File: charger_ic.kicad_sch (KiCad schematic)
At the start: 1 part, among them U8 BQ25731RSNR

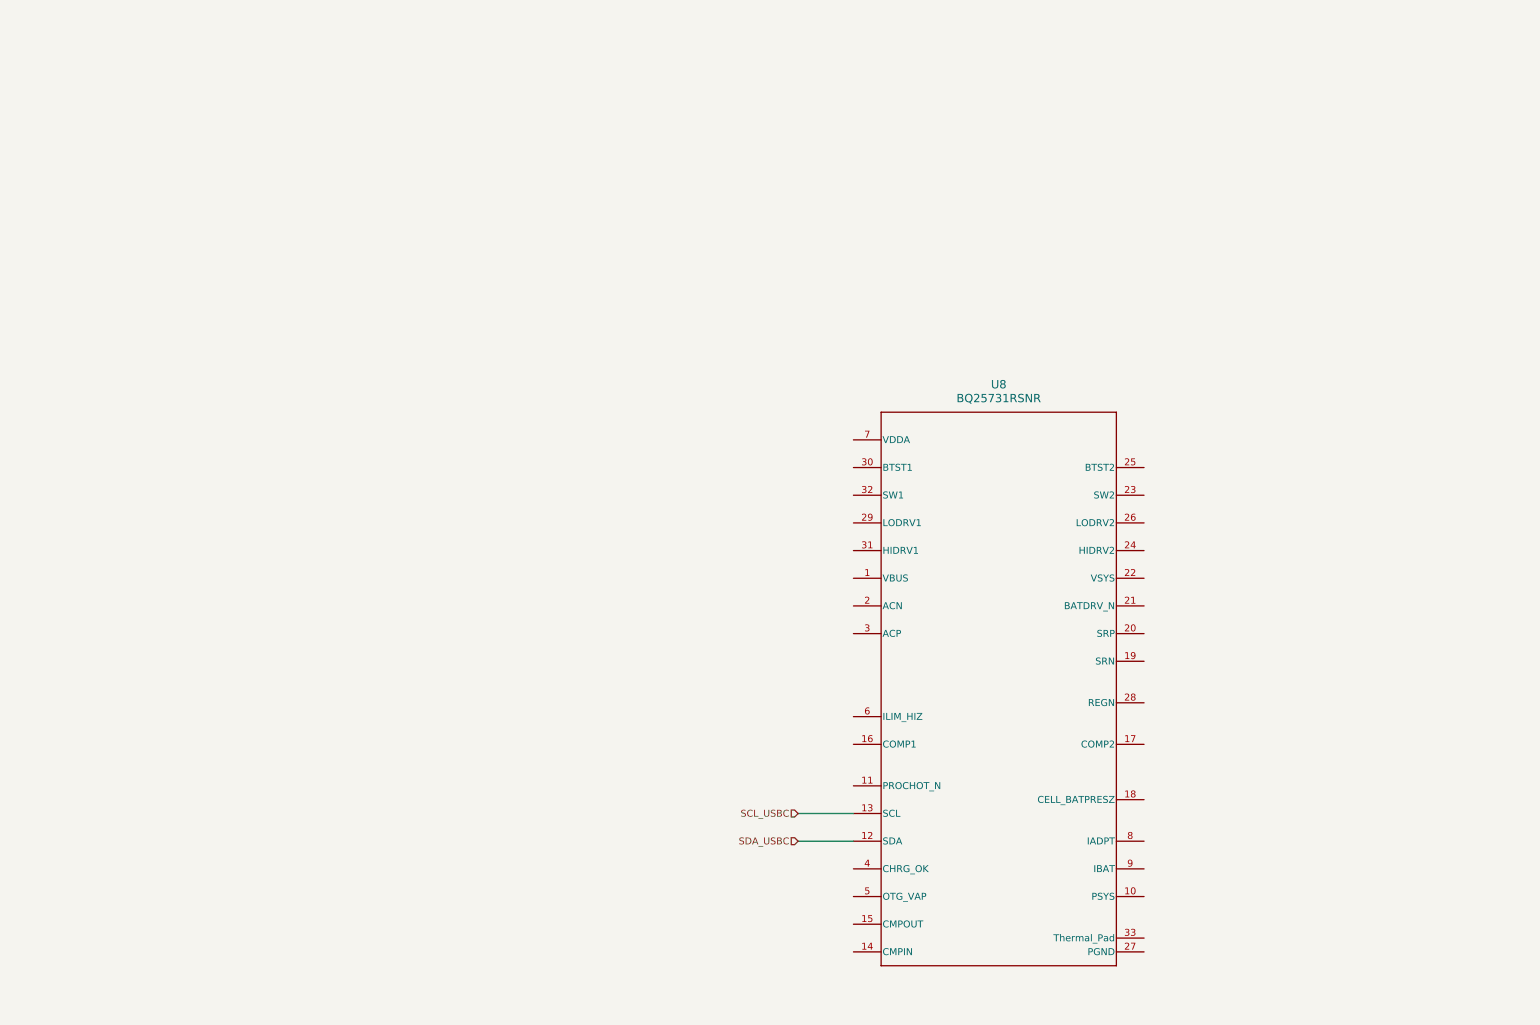
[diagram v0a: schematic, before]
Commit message: adding charging stages finally
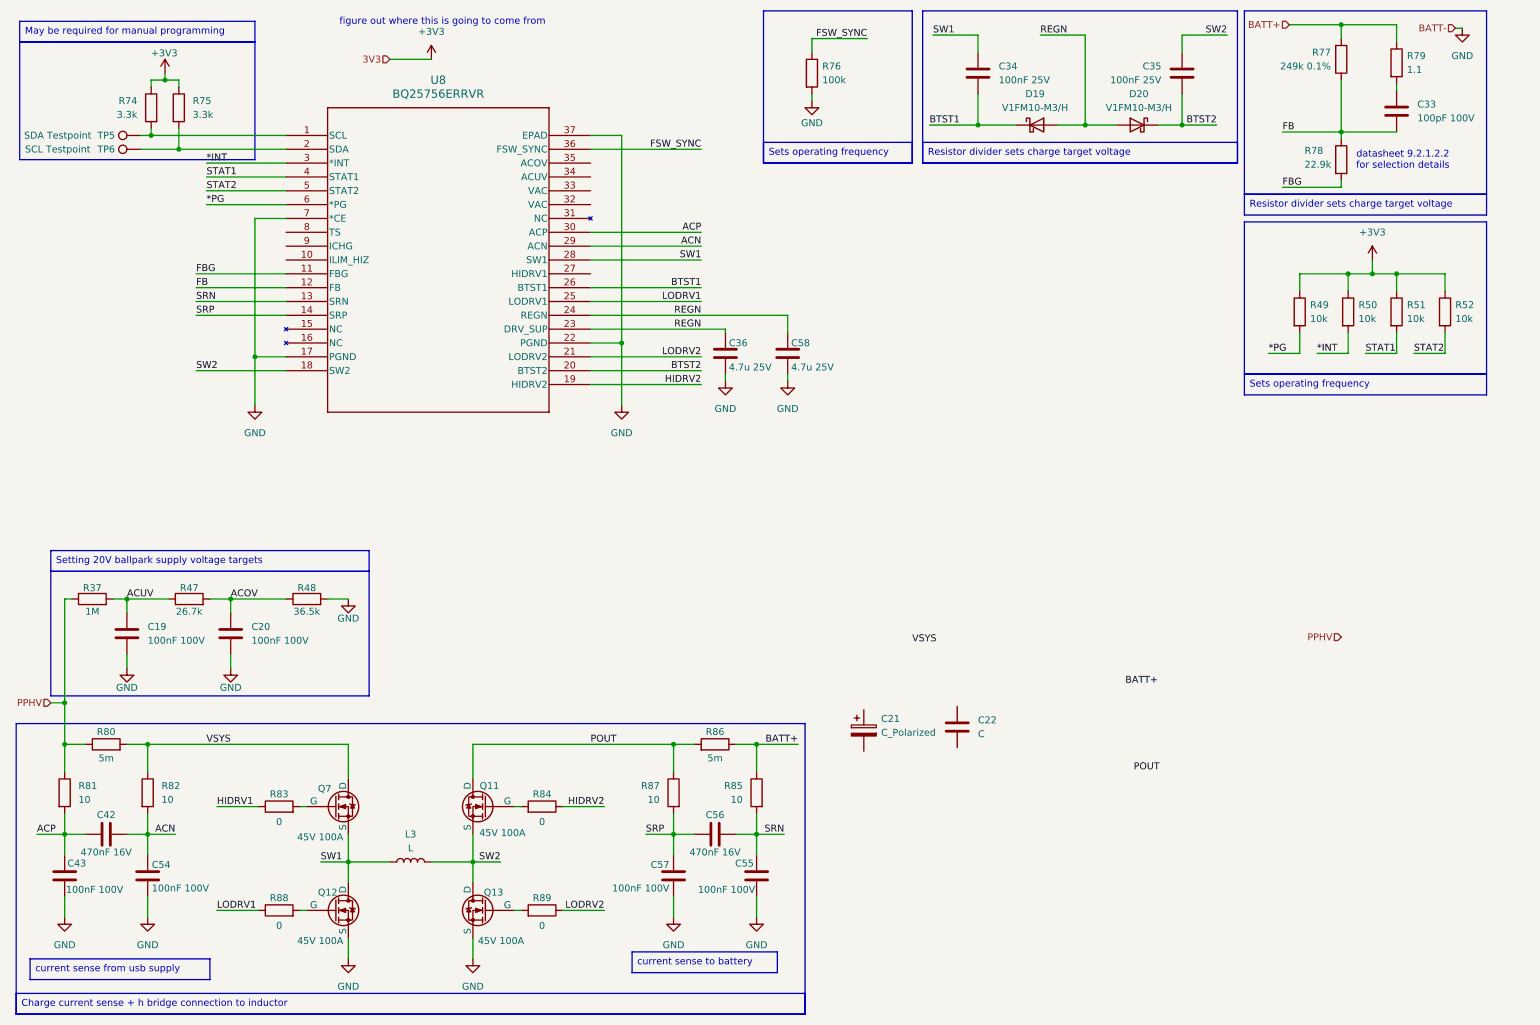
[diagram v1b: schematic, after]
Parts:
- removed U8: BQ25731RSNR, RSN0032B-IPC_A, symbol BQ25731:BQ25731RSNR
- added C19, C20, C43, C54, C55, C57: 100nF 100V, symbol Device:C
- added C21: C_Polarized, symbol Device:C_Polarized
- added C22: C, symbol Device:C
- added C33: 100pF 100V, symbol Device:C
- added C34, C35: 100nF 25V, symbol Device:C
- added C36, C58: 4.7u 25V, symbol Device:C
- added C42, C56: 470nF 16V, symbol Device:C
- added D19, D20: V1FM10-M3/H, symbol Device:D_Schottky
- added L3: L, symbol Device:L
- added Q11, Q12, Q13, Q7: 45V 100A, symbol Simulation_SPICE:NMOS
- added R37: 1M, symbol Device:R
- added R47: 26.7k, symbol Device:R
- added R48: 36.5k, symbol Device:R
- added R49, R50, R51, R52: 10k, symbol Device:R
- added R74, R75: 3.3k, symbol Device:R
- added R76: 100k, symbol Device:R
- added R77: 249k 0.1%, symbol Device:R
- added R78: 22.9k, symbol Device:R
- added R79: 1.1, symbol Device:R
- added R80, R86: 5m, symbol Device:R
- added R81, R82, R85, R87: 10, symbol Device:R
- added R83, R84, R88, R89: 0, symbol Device:R
- added TP5: SDA Testpoint, symbol Connector:TestPoint
- added TP6: SCL Testpoint, symbol Connector:TestPoint
- added U8: BQ25756ERRVR, VQFN36_RRV_TEX, symbol BQ25756E:BQ25756ERRVR
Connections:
- new net: Q7.2 (G), R83.2
- new net: R74.2, TP5.1, U8.1 (SCL)
- new net: Q12.2 (G), R88.2
- new net: Q11.2 (G), R84.2
- new net: C33.1, R79.2
- new net: Q13.2 (G), R89.2
- new net: R75.2, TP6.1, U8.2 (SDA)
- new net *INT: R50.2, U8.3 (*INT)
- new net *PG: R49.2, U8.6 (*PG)
- new net +3V3: R49.1, R50.1, R51.1, R52.1, R74.1, R75.1
- new net ACN: C42.2, C54.1, R82.2, U8.29 (ACN)
- new net ACOV: C20.1, R47.2, R48.1
- new net ACP: C42.1, C43.1, R81.2, U8.30 (ACP)
- new net ACUV: C19.1, R37.2, R47.1
- new net BATT+: R77.2, R79.1, R85.1, R86.1
- new net BTST1: C34.1, D19.1 (K), U8.26 (BTST1)
- new net BTST2: C35.1, D20.1 (K), U8.20 (BTST2)
- new net FB: C33.2, R77.1, R78.1, U8.12 (FB)
- new net FBG: R78.2, U8.11 (FBG)
- new net FSW_SYNC: R76.1, U8.36 (FSW_SYNC)
- new net GND: C19.2, C20.2, C36.2, C43.2, C54.2, C55.2, C57.2, C58.2, Q12.3 (S), Q13.3 (S), R48.2, R76.2, U8.17 (PGND), U8.22 (PGND), U8.37 (EPAD), U8.7 (*CE)
- new net HIDRV1: R83.1
- new net HIDRV2: R84.1, U8.19 (HIDRV2)
- new net LODRV1: R88.1, U8.25 (LODRV1)
- new net LODRV2: R89.1, U8.21 (LODRV2)
- new net POUT: Q11.1 (D), R86.2, R87.1
- new net PPHV: R37.1, R80.1, R81.1
- new net REGN: C36.1, C58.1, D19.2 (A), D20.2 (A), U8.23 (DRV_SUP), U8.24 (REGN)
- new net SRN: C55.1, C56.1, R85.2, U8.13 (SRN)
- new net SRP: C56.2, C57.1, R87.2, U8.14 (SRP)
- new net STAT1: R51.2, U8.4 (STAT1)
- new net STAT2: R52.2, U8.5 (STAT2)
- new net SW1: C34.2, L3.1, Q12.1 (D), Q7.3 (S), U8.28 (SW1)
- new net SW2: C35.2, L3.2, Q11.3 (S), Q13.1 (D), U8.18 (SW2)
- new net VSYS: Q7.1 (D), R80.2, R82.1
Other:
- note added: "datasheet 9.2.1.2.2 for selection details"
- note added: "figure out where this is going to come from"
